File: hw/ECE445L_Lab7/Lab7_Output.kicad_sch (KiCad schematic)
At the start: 33 parts, among them M1 Motor _DC, M2 Motor _DC, M3 Motor _DC, M4 Motor _DC, M7 Solenoid_DC, Q1 NTR4501NT1G, Q2 NTR4501NT1G, Q3 NTR4501NT1G, Q4 NTR4501NT1G, Q5 NTR4501NT1G, Q6 NTR4501NT1G, Q7 NTR4501NT1G, Q8 NTR4501NT1G, Q9 NTR4501NT1G, U2 Adafruit ST7735R, U5 HiLetGo_ST7735R

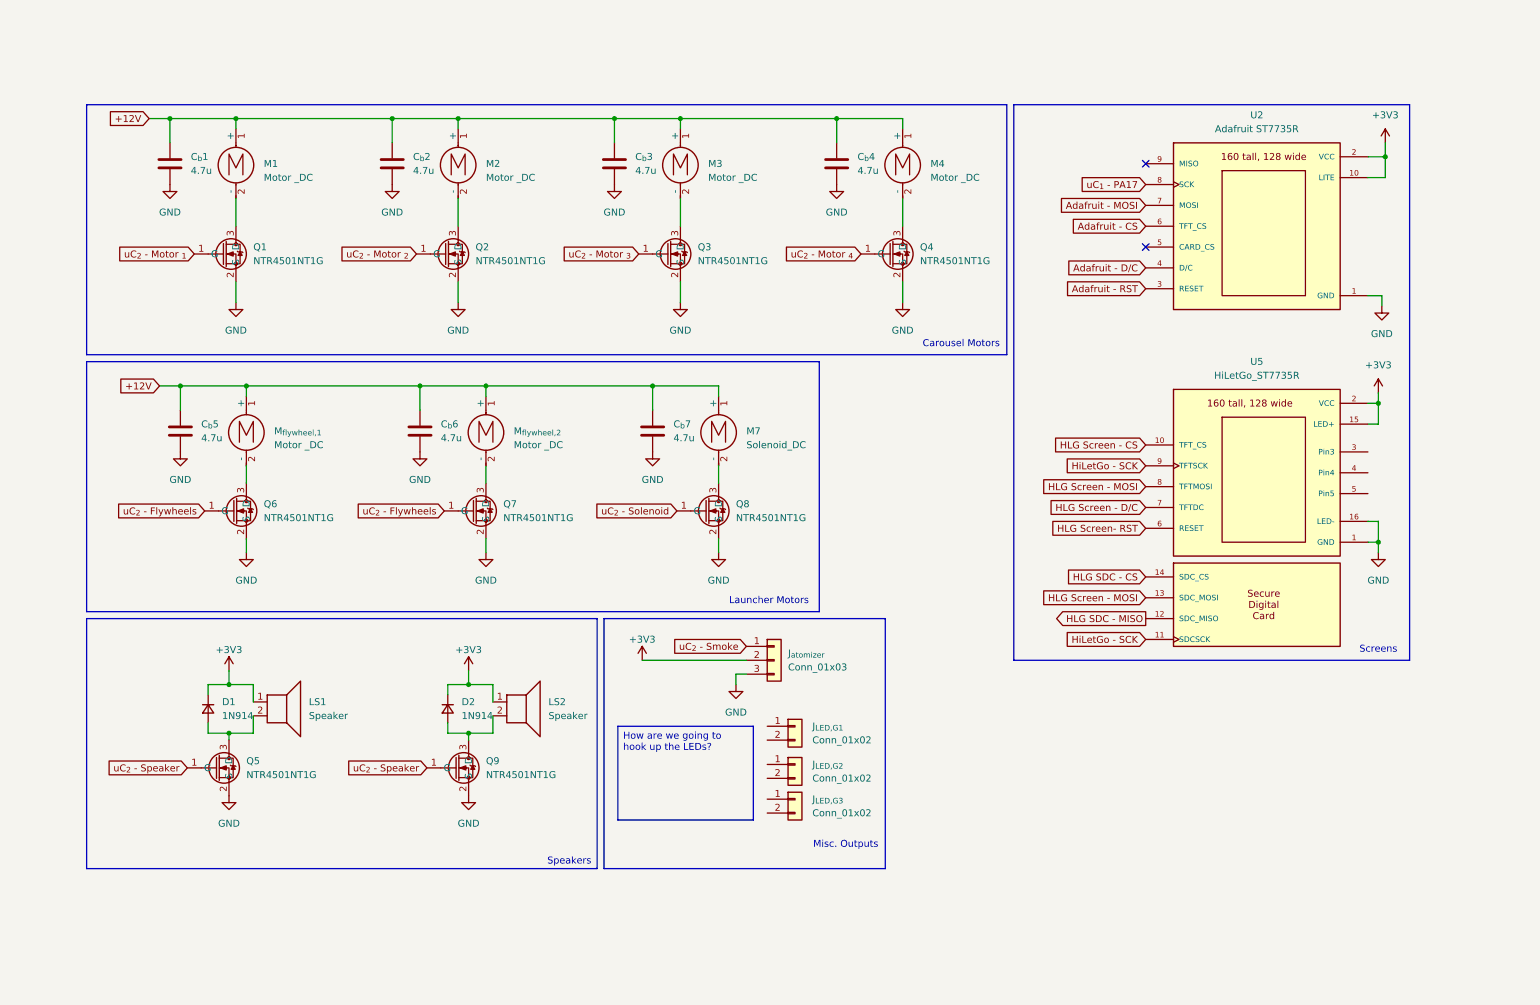
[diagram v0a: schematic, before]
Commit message: finished prelim schem
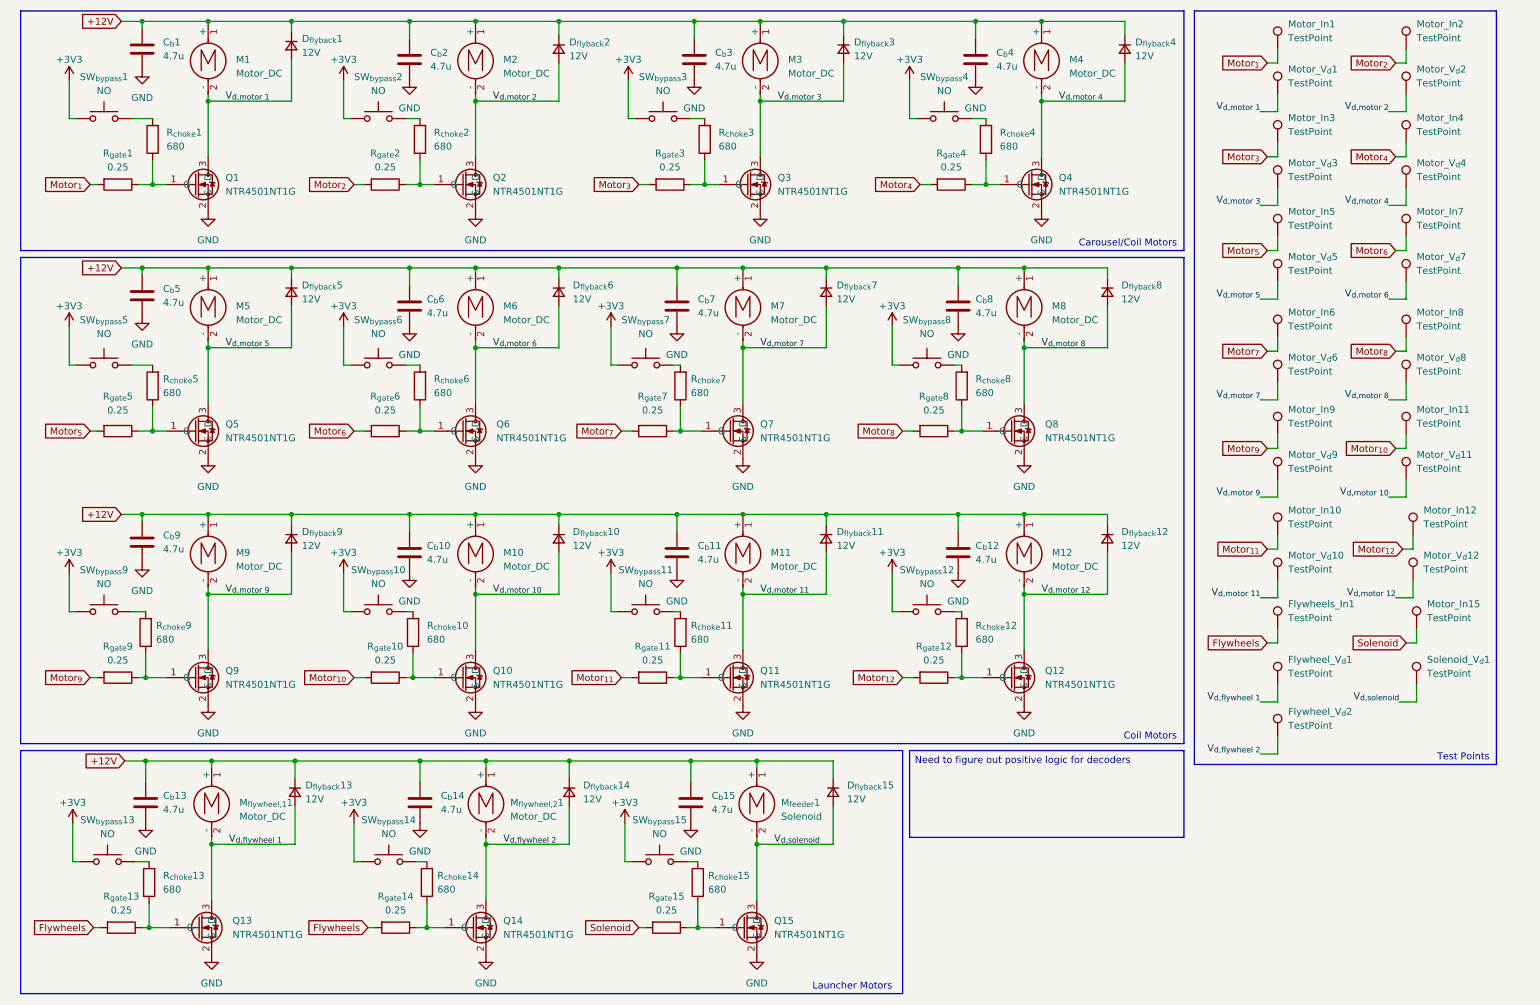
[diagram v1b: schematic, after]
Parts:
- removed D1, D2: 1N914, Diode_THT:D_5W_P12.70mm_Horizontal, symbol Device:D_Small
- removed J_{LED,G1}, J_{LED,G2}, J_{LED,G3}: Conn_01x02, Connector_PinSocket_2.54mm:PinSocket_1x02_P2.54mm_Vertical, symbol Connector_Generic:Conn_01x02
- removed J_{atomizer}: Conn_01x03, Connector_PinSocket_2.54mm:PinSocket_1x03_P2.54mm_Vertical, symbol Connector_Generic:Conn_01x03
- removed LS1, LS2: Speaker, ECE445L:PinHeader_1x02_P2.54mm_Vertical, symbol ECE445L:Speaker
- removed U2: Adafruit ST7735R, ECE445L:adafruit_st7735r2, symbol ECE445L:Adafruit_ST7735R
- removed U5: HiLetGo_ST7735R, ECE445L:hiletgo_st7735r2, symbol ECE445L:HiLetGo_ST7735R
- added C_{b}10, C_{b}11, C_{b}12, C_{b}5, C_{b}6, C_{b}7, C_{b}8, C_{b}9: 4.7u, Capacitor_SMD:C_0603_1608Metric_Pad1.08x0.95mm_HandSolder, symbol ECE445L:C
- added D_{flyback}1, D_{flyback}10, D_{flyback}11, D_{flyback}12, D_{flyback}13, D_{flyback}14, D_{flyback}15, D_{flyback}2, D_{flyback}3, D_{flyback}4, D_{flyback}5, D_{flyback}6, D_{flyback}7, D_{flyback}8, D_{flyback}9: 12V, Diode_SMD:D_SOD-523, symbol Device:D_Small
- added Flywheel_V_{d}1, Flywheel_V_{d}2, Flywheels_In1, Motor_In1, Motor_In10, Motor_In11, Motor_In12, Motor_In15, Motor_In2, Motor_In3, Motor_In4, Motor_In5, Motor_In6, Motor_In7, Motor_In8, Motor_In9, Motor_V_{d}1, Motor_V_{d}10, Motor_V_{d}11, Motor_V_{d}12, Motor_V_{d}2, Motor_V_{d}3, Motor_V_{d}4, Motor_V_{d}5, Motor_V_{d}6, Motor_V_{d}7, Motor_V_{d}8, Motor_V_{d}9, Solenoid_V_{d}1: TestPoint, TestPoint:TestPoint_Keystone_5010-5014_Multipurpose, symbol Connector:TestPoint
- added M10, M11, M12, M5, M6, M7, M8, M9: Motor_DC, Connector_AMASS:AMASS_XT30U-M_1x02_P5.0mm_Vertical, symbol Motor:Motor_DC
- added Q10, Q11, Q12, Q6, Q7, Q8: NTR4501NT1G, ECE445L:SOT96P237X111-3N, symbol ECE445L:NTR4501NT1G
- added R_{choke}1, R_{choke}10, R_{choke}11, R_{choke}12, R_{choke}13, R_{choke}14, R_{choke}15, R_{choke}2, R_{choke}3, R_{choke}4, R_{choke}5, R_{choke}6, R_{choke}7, R_{choke}8, R_{choke}9: 680, Resistor_SMD:R_0603_1608Metric_Pad0.98x0.95mm_HandSolder, symbol Device:R
- added R_{gate}1, R_{gate}10, R_{gate}11, R_{gate}12, R_{gate}13, R_{gate}14, R_{gate}15, R_{gate}2, R_{gate}3, R_{gate}4, R_{gate}5, R_{gate}6, R_{gate}7, R_{gate}8, R_{gate}9: 0.25, Resistor_SMD:R_0603_1608Metric_Pad0.98x0.95mm_HandSolder, symbol Device:R
- added SW_{bypass}1, SW_{bypass}10, SW_{bypass}11, SW_{bypass}12, SW_{bypass}13, SW_{bypass}14, SW_{bypass}15, SW_{bypass}2, SW_{bypass}3, SW_{bypass}4, SW_{bypass}5, SW_{bypass}6, SW_{bypass}7, SW_{bypass}8, SW_{bypass}9: NO, ECE445L:SW_PUSH_6mm, symbol ECE445L:SW_Push
- C_{b}1, C_{b}2, C_{b}3, C_{b}4: footprint Capacitor_SMD:C_0805_2012Metric_Pad1.18x1.45mm_HandSolder -> Capacitor_SMD:C_0603_1608Metric_Pad1.08x0.95mm_HandSolder; Distributor (none) -> Mouser; Manufacturer (none) -> Walsin; Manufacturer_Part_Number (none) -> 0805X475M250CT; Mouser Part Number (none) -> 791-0805X475M250CT
- C_{b}13: renamed from C_{b}5; footprint Capacitor_SMD:C_0805_2012Metric_Pad1.18x1.45mm_HandSolder -> Capacitor_SMD:C_0603_1608Metric_Pad1.08x0.95mm_HandSolder; Distributor (none) -> Mouser; Manufacturer (none) -> Walsin; Manufacturer_Part_Number (none) -> 0805X475M250CT; Mouser Part Number (none) -> 791-0805X475M250CT
- C_{b}14: renamed from C_{b}6; footprint Capacitor_SMD:C_0805_2012Metric_Pad1.18x1.45mm_HandSolder -> Capacitor_SMD:C_0603_1608Metric_Pad1.08x0.95mm_HandSolder; Distributor (none) -> Mouser; Manufacturer (none) -> Walsin; Manufacturer_Part_Number (none) -> 0805X475M250CT; Mouser Part Number (none) -> 791-0805X475M250CT
- C_{b}15: renamed from C_{b}7; footprint Capacitor_SMD:C_0805_2012Metric_Pad1.18x1.45mm_HandSolder -> Capacitor_SMD:C_0603_1608Metric_Pad1.08x0.95mm_HandSolder; Distributor (none) -> Mouser; Manufacturer (none) -> Walsin; Manufacturer_Part_Number (none) -> 0805X475M250CT; Mouser Part Number (none) -> 791-0805X475M250CT
- M1, M2, M3, M4: value Motor _DC -> Motor_DC; footprint Connector_JST:JST_PH_B2B-PH-K_1x02_P2.00mm_Vertical -> Connector_AMASS:AMASS_XT30U-M_1x02_P5.0mm_Vertical; Distributor (none) -> Amazon; Manufacturer (none) -> Coliao
- M_{feeder}1: renamed from M7; value Solenoid_DC -> Solenoid; Distributor (none) -> Amazon; Manufacturer (none) -> Heschen
- M_{flywheel,1}1: renamed from M_{flywheel,1}; value Motor _DC -> Motor_DC; footprint Connector_JST:JST_PH_B2B-PH-K_1x02_P2.00mm_Vertical -> Connector_AMASS:AMASS_XT30U-M_1x02_P5.0mm_Vertical; Distributor (none) -> Amazon; Manufacturer (none) -> AUTOTOOLHOME
- M_{flywheel,2}1: renamed from M_{flywheel,2}; value Motor _DC -> Motor_DC; footprint Connector_JST:JST_PH_B2B-PH-K_1x02_P2.00mm_Vertical -> Connector_AMASS:AMASS_XT30U-M_1x02_P5.0mm_Vertical; Distributor (none) -> Amazon; Manufacturer (none) -> AUTOTOOLHOME
- Q1, Q2, Q3, Q4, Q5, Q9: Distributor (none) -> Checkout; Manufacturer (none) -> onsemi
- Q13: renamed from Q6; Distributor (none) -> Checkout; Manufacturer (none) -> onsemi
- Q14: renamed from Q7; Distributor (none) -> Checkout; Manufacturer (none) -> onsemi
- Q15: renamed from Q8; Distributor (none) -> Checkout; Manufacturer (none) -> onsemi
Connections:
- net +12V: now also C_{b}10.1, C_{b}11.1, C_{b}12.1, C_{b}5.1, C_{b}6.1, C_{b}7.1, C_{b}8.1, C_{b}9.1, D_{flyback}1.1 (K), D_{flyback}10.1 (K), D_{flyback}11.1 (K), D_{flyback}12.1 (K), D_{flyback}13.1 (K), D_{flyback}14.1 (K), D_{flyback}15.1 (K), D_{flyback}2.1 (K), D_{flyback}3.1 (K), D_{flyback}4.1 (K), D_{flyback}5.1 (K), D_{flyback}6.1 (K), D_{flyback}7.1 (K), D_{flyback}8.1 (K), D_{flyback}9.1 (K), M10.1 (+), M11.1 (+), M12.1 (+), M5.1 (+), M6.1 (+), M7.1 (+), M8.1 (+), M9.1 (+)
- net +3V3: now also SW_{bypass}1.1, SW_{bypass}10.1, SW_{bypass}11.1, SW_{bypass}12.1, SW_{bypass}13.1, SW_{bypass}14.1, SW_{bypass}15.1, SW_{bypass}2.1, SW_{bypass}3.1, SW_{bypass}4.1, SW_{bypass}5.1, SW_{bypass}6.1, SW_{bypass}7.1, SW_{bypass}8.1, SW_{bypass}9.1
- net GND: now also C_{b}10.2, C_{b}11.2, C_{b}12.2, C_{b}5.2, C_{b}6.2, C_{b}7.2, C_{b}8.2, C_{b}9.2, Q10.2 (S), Q11.2 (S), Q12.2 (S), Q6.2 (S), Q7.2 (S), Q8.2 (S)
- net V_{d,motor 5}: now reaches Q5.3 (D)
- net V_{d,motor 5}: now also D_{flyback}5.2 (A), M5.2 (-), Motor_V_{d}5.1
- net V_{d,motor 3}: now reaches M3.2 (-), Q3.3 (D)
- net V_{d,motor 3}: now also D_{flyback}3.2 (A), Motor_V_{d}3.1
- net V_{d,motor 9}: now reaches Q9.3 (D)
- net V_{d,motor 9}: now also D_{flyback}9.2 (A), M9.2 (-), Motor_V_{d}9.1
- net V_{d,solenoid}: now reaches M_{feeder}1.2 (-), Q15.3 (D)
- net V_{d,solenoid}: now also D_{flyback}15.2 (A), Solenoid_V_{d}1.1
- net V_{d,flywheel 2}: now reaches M_{flywheel,2}1.2 (-), Q14.3 (D)
- net V_{d,flywheel 2}: now also D_{flyback}14.2 (A), Flywheel_V_{d}2.1
- net V_{d,motor 4}: now reaches M4.2 (-), Q4.3 (D)
- net V_{d,motor 4}: now also D_{flyback}4.2 (A), Motor_V_{d}4.1
- net V_{d,motor 2}: now reaches M2.2 (-), Q2.3 (D)
- net V_{d,motor 2}: now also D_{flyback}2.2 (A), Motor_V_{d}2.1
- net V_{d,motor 1}: now reaches M1.2 (-), Q1.3 (D)
- net V_{d,motor 1}: now also D_{flyback}1.2 (A), Motor_V_{d}1.1
- net V_{d,flywheel 1}: now reaches M_{flywheel,1}1.2 (-), Q13.3 (D)
- net V_{d,flywheel 1}: now also D_{flyback}13.2 (A), Flywheel_V_{d}1.1
- net uC_{2} - Flywheels: no longer names the net of Q14.1 (G)
- net uC_{2} - Flywheels: now also R_{choke}14.1, R_{gate}14.1; no longer Q13.1 (G)
- net uC_{2} - Motor _{1}: no longer names the net of Q1.1 (G)
- net uC_{2} - Motor _{1}: now also R_{choke}1.1, R_{gate}1.1
- net uC_{2} - Motor _{2}: no longer names the net of Q2.1 (G)
- net uC_{2} - Motor _{2}: now also R_{choke}2.1, R_{gate}2.1
- net uC_{2} - Motor _{3}: no longer names the net of Q3.1 (G)
- net uC_{2} - Motor _{3}: now also R_{choke}3.1, R_{gate}3.1
- net uC_{2} - Motor _{4}: no longer names the net of Q4.1 (G)
- net uC_{2} - Motor _{4}: now also R_{choke}4.1, R_{gate}4.1
- net uC_{2} - Solenoid: no longer names the net of Q15.1 (G)
- net uC_{2} - Solenoid: now also R_{choke}15.1, R_{gate}15.1
- net uC_{2} - Speaker: no longer names the net of Q5.1 (G)
- net uC_{2} - Speaker: now also R_{choke}5.1, R_{gate}5.1; no longer Q9.1 (G)
- new net: Q11.1 (G), R_{choke}11.1, R_{gate}11.1
- new net: R_{choke}6.2, SW_{bypass}6.2
- new net: Q8.1 (G), R_{choke}8.1, R_{gate}8.1
- new net: Q10.1 (G), R_{choke}10.1, R_{gate}10.1
- new net: R_{choke}2.2, SW_{bypass}2.2
- new net: Q6.1 (G), R_{choke}6.1, R_{gate}6.1
- new net: Q12.1 (G), R_{choke}12.1, R_{gate}12.1
- new net: R_{choke}4.2, SW_{bypass}4.2
- new net: R_{choke}9.2, SW_{bypass}9.2
- new net: Q7.1 (G), R_{choke}7.1, R_{gate}7.1
- new net: Q9.1 (G), R_{choke}9.1, R_{gate}9.1
- new net: R_{choke}11.2, SW_{bypass}11.2
- new net: R_{choke}5.2, SW_{bypass}5.2
- new net: R_{choke}14.2, SW_{bypass}14.2
- new net: R_{choke}15.2, SW_{bypass}15.2
- new net: R_{choke}7.2, SW_{bypass}7.2
- new net: R_{choke}3.2, SW_{bypass}3.2
- new net: R_{choke}12.2, SW_{bypass}12.2
- new net: R_{choke}10.2, SW_{bypass}10.2
- new net: Q13.1 (G), R_{choke}13.1, R_{gate}13.1
- new net: R_{choke}8.2, SW_{bypass}8.2
- new net: R_{choke}1.2, SW_{bypass}1.2
- new net: R_{choke}13.2, SW_{bypass}13.2
- new net Flywheels: Flywheels_In1.1, R_{gate}13.2, R_{gate}14.2
- new net Motor_{10}: Motor_In11.1, R_{gate}10.2
- new net Motor_{11}: Motor_In10.1, R_{gate}11.2
- new net Motor_{12}: Motor_In12.1, R_{gate}12.2
- new net Motor_{1}: Motor_In1.1, R_{gate}1.2
- new net Motor_{2}: Motor_In2.1, R_{gate}2.2
- new net Motor_{3}: Motor_In3.1, R_{gate}3.2
- new net Motor_{4}: Motor_In4.1, R_{gate}4.2
- new net Motor_{5}: Motor_In5.1, R_{gate}5.2
- new net Motor_{6}: Motor_In7.1, R_{gate}6.2
- new net Motor_{7}: Motor_In6.1, R_{gate}7.2
- new net Motor_{8}: Motor_In8.1, R_{gate}8.2
- new net Motor_{9}: Motor_In9.1, R_{gate}9.2
- new net Solenoid: Motor_In15.1, R_{gate}15.2
- new net V_{d,motor 10}: D_{flyback}10.2 (A), M10.2 (-), Motor_V_{d}11.1, Q10.3 (D)
- new net V_{d,motor 11}: D_{flyback}11.2 (A), M11.2 (-), Motor_V_{d}10.1, Q11.3 (D)
- new net V_{d,motor 12}: D_{flyback}12.2 (A), M12.2 (-), Motor_V_{d}12.1, Q12.3 (D)
- new net V_{d,motor 6}: D_{flyback}6.2 (A), M6.2 (-), Motor_V_{d}7.1, Q6.3 (D)
- new net V_{d,motor 7}: D_{flyback}7.2 (A), M7.2 (-), Motor_V_{d}6.1, Q7.3 (D)
- new net V_{d,motor 8}: D_{flyback}8.2 (A), M8.2 (-), Motor_V_{d}8.1, Q8.3 (D)
- no-connect marks 2 -> 0
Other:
- note added: "Carousel/Coil Motors"
- note added: "Coil Motors"
- note added: "Test Points"
- note removed: "Carousel Motors"
- note removed: "Misc. Outputs"
- note removed: "Screens"
- note removed: "Speakers"
- moved on the sheet: C_{b}1, C_{b}13, C_{b}14, C_{b}15, C_{b}2, C_{b}3, C_{b}4, M1, M2, M3, M4, M_{feeder}1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
